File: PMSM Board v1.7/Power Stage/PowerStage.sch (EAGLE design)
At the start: 16 parts, among them U1 TPS73733-Q1_DRB_8, U2 TPS54240_DRC_10, U3 LP38692_NGG_6

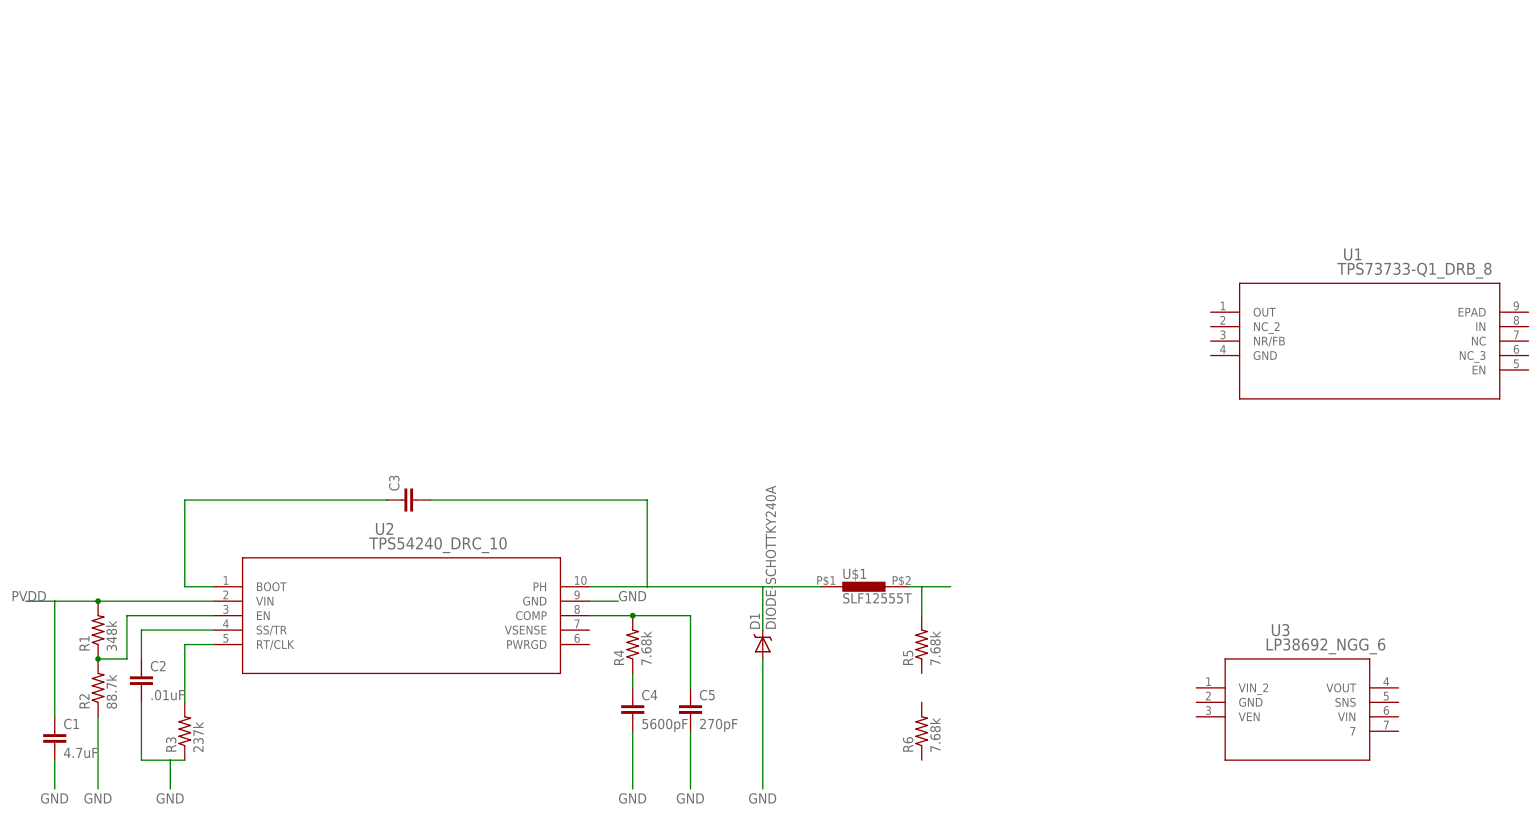
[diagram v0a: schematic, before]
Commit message: More switcher work.
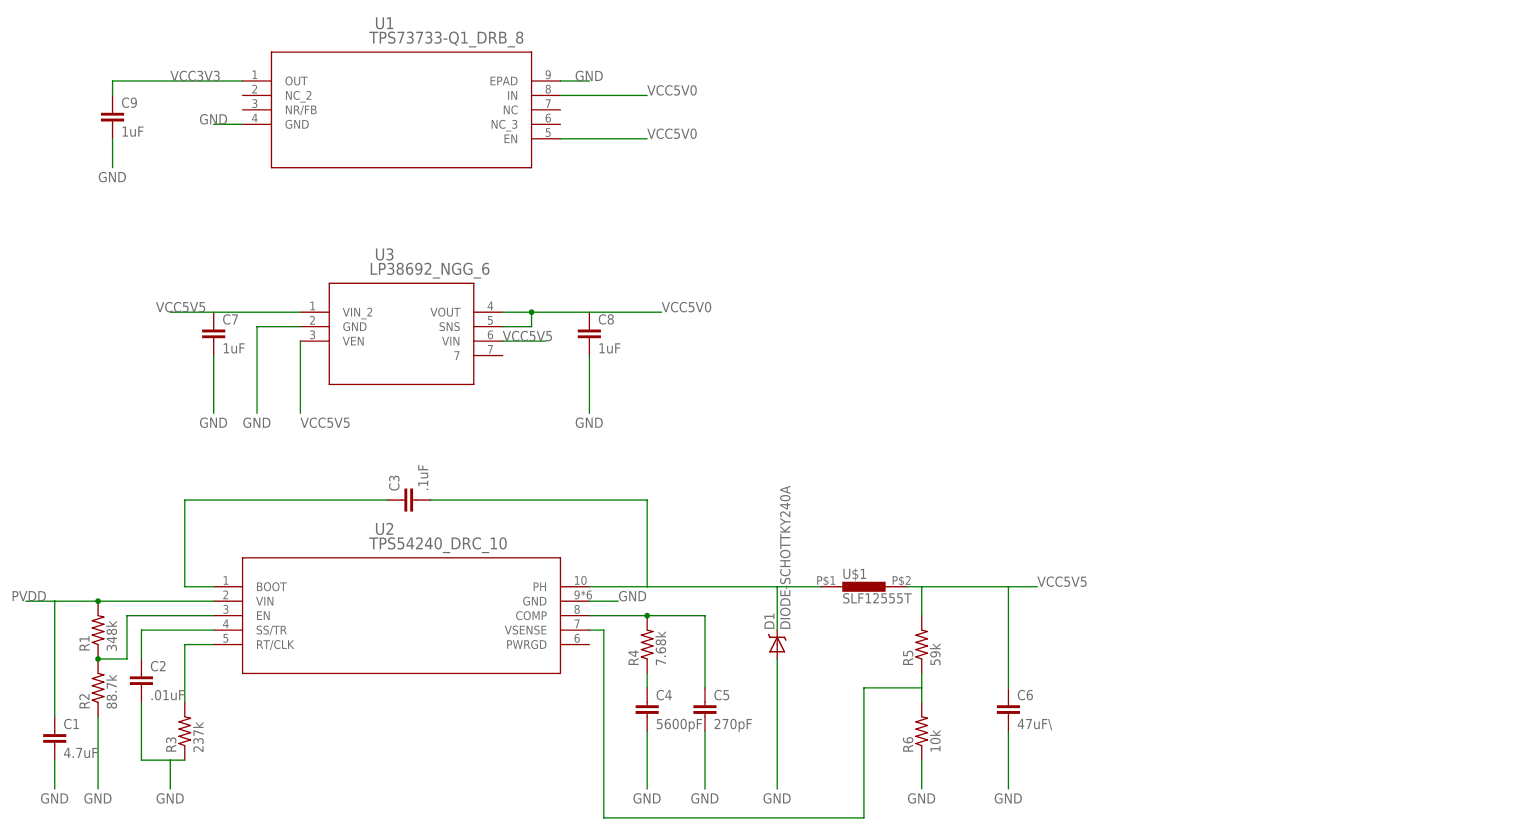
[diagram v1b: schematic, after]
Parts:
- added C6: 47uF\, SwitcherPowerStage:CAP
- added C7, C8, C9: 1uF, SwitcherPowerStage:CAP0805
- C3: value (none) -> .1uF
- C4, C5: device SwitcherPowerStage:CAP1210 -> SwitcherPowerStage:CAP0805
- R5: value 7.68k -> 59k
- R6: value 7.68k -> 10k
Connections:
- removed net N$8: R5.2, U$1.2
- new net N$9: R5.1, R6.2, U2.VSENSE
- new net VCC3V3: C9.1, U1.OUT
- new net VCC5V0: U1.EN, U1.IN, U3.SNS, U3.VOUT
- new net VCC5V5: C6.1, R5.2, U$1.2, U3.VEN, U3.VIN, U3.VIN_2
- net GND: now also C6.2, C7.2, C8.2, C9.2, R6.1, U1.EPAD, U1.GND, U3.GND
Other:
- moved on the sheet: C4, C5, D1, R4, U1, U2, U3
